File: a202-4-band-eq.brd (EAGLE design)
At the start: 100 x 50 mm, 71 parts, among them U1 SCREW-M2X8, U10 FX2-20S-1.27DS, U2 SCREW-M2X8, U3 NUT-M2-SELFLOCK, U4 NUT-M2-SELFLOCK, U5 FX2-20P-1.27DS, U6 SCREW-M2X8, U7 SCREW-M2X8, U8 NUT-M2-SELFLOCK, U9 NUT-M2-SELFLOCK

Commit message: Add Potentiometer Knobs
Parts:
- added O1, O2, O3, O4: 450-AA150(15MM,D,BLACK), hardware:EMPTY
- added O5, O6, O7, O8: 450-CP153(15MM,BLUE/WHITE), hardware:EMPTY
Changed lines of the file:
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@@
 <attribute name="MOUSER" value="81-RCER71H104K0A2H3B" x="12" y="-171" size="1.778" layer="27" display="off"/>
+</element>
+<element name="O1" library="hardware" package="EMPTY" value="450-AA150(15MM,D,BLACK)" x="-8" y="-109.25">
+<attribute name="MOUSER" value="450-AA150" x="-8" y="-109.25" size="1.778" layer="27" display="off"/>
+</element>
+<element name="O2" library="hardware" package="EMPTY" value="450-AA150(15MM,D,BLACK)" x="-9" y="-110.5">
+<attribute name="MOUSER" value="450-AA150" x="-9" y="-110.5" size="1.778" layer="27" display="off"/>
+</element>
+<element name="O3" library="hardware" package="EMPTY" value="450-AA150(15MM,D,BLACK)" x="-10" y="-111.75">
+<attribute name="MOUSER" value="450-AA150" x="-10" y="-111.75" size="1.778" layer="27" display="off"/>
+</element>
+<element name="O4" library="hardware" package="EMPTY" value="450-AA150(15MM,D,BLACK)" x="-11" y="-113">
+<attribute name="MOUSER" value="450-AA150" x="-11" y="-113" size="1.778" layer="27" display="off"/>
+</element>
+<element name="O5" library="hardware" package="EMPTY" value="450-CP153(15MM,BLUE/WHITE)" x="-12" y="-114.25">
+<attribute name="MOUSER" value="450-CP153" x="-12" y="-114.25" size="1.778" layer="27" display="off"/>
+</element>
+<element name="O6" library="hardware" package="EMPTY" value="450-CP153(15MM,BLUE/WHITE)" x="-13" y="-115.5">
+<attribute name="MOUSER" value="450-CP153" x="-13" y="-115.5" size="1.778" layer="27" display="off"/>
+</element>
+<element name="O7" library="hardware" package="EMPTY" value="450-CP153(15MM,BLUE/WHITE)" x="-14" y="-116.75">
+<attribute name="MOUSER" value="450-CP153" x="-14" y="-116.75" size="1.778" layer="27" display="off"/>
+</element>
+<element name="O8" library="hardware" package="EMPTY" value="450-CP153(15MM,BLUE/WHITE)" x="-15" y="-118">
+<attribute name="MOUSER" value="450-CP153" x="-15" y="-118" size="1.778" layer="27" display="off"/>
 </element>
 </elements>

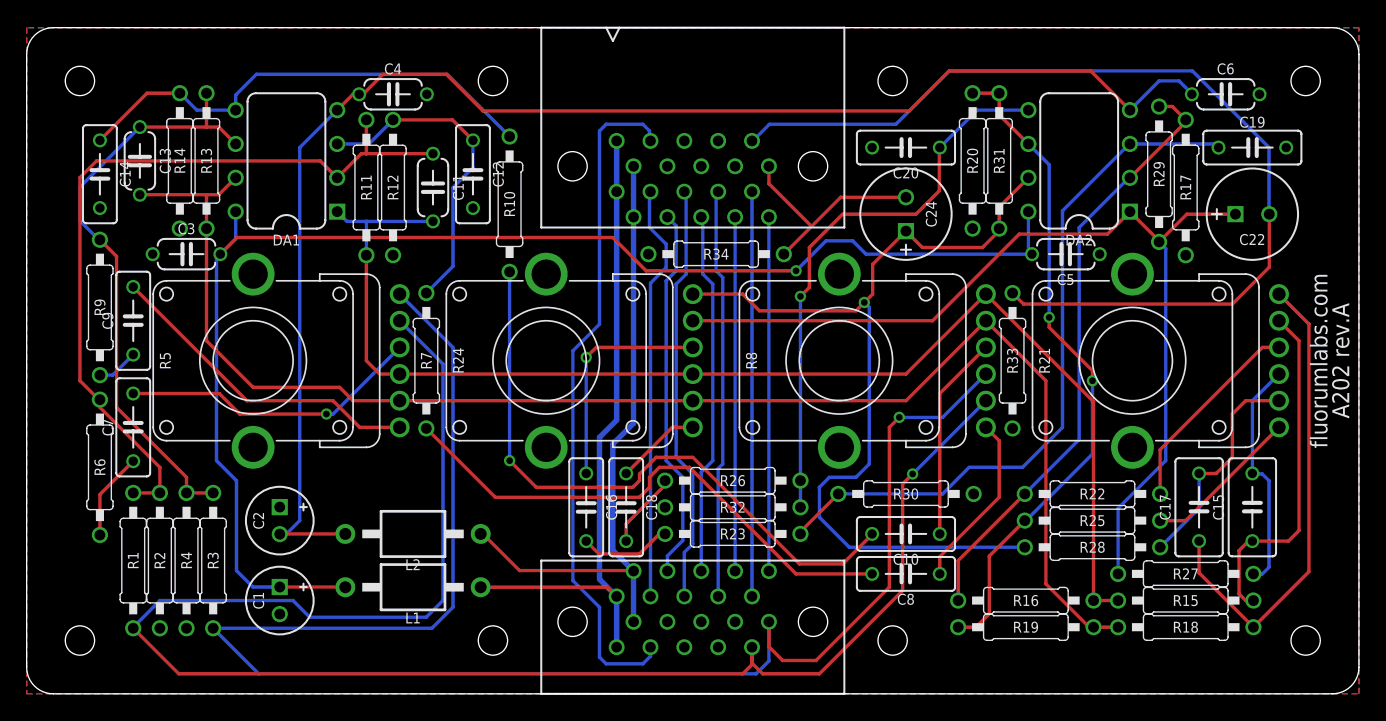
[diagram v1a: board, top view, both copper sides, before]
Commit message: PCB Update
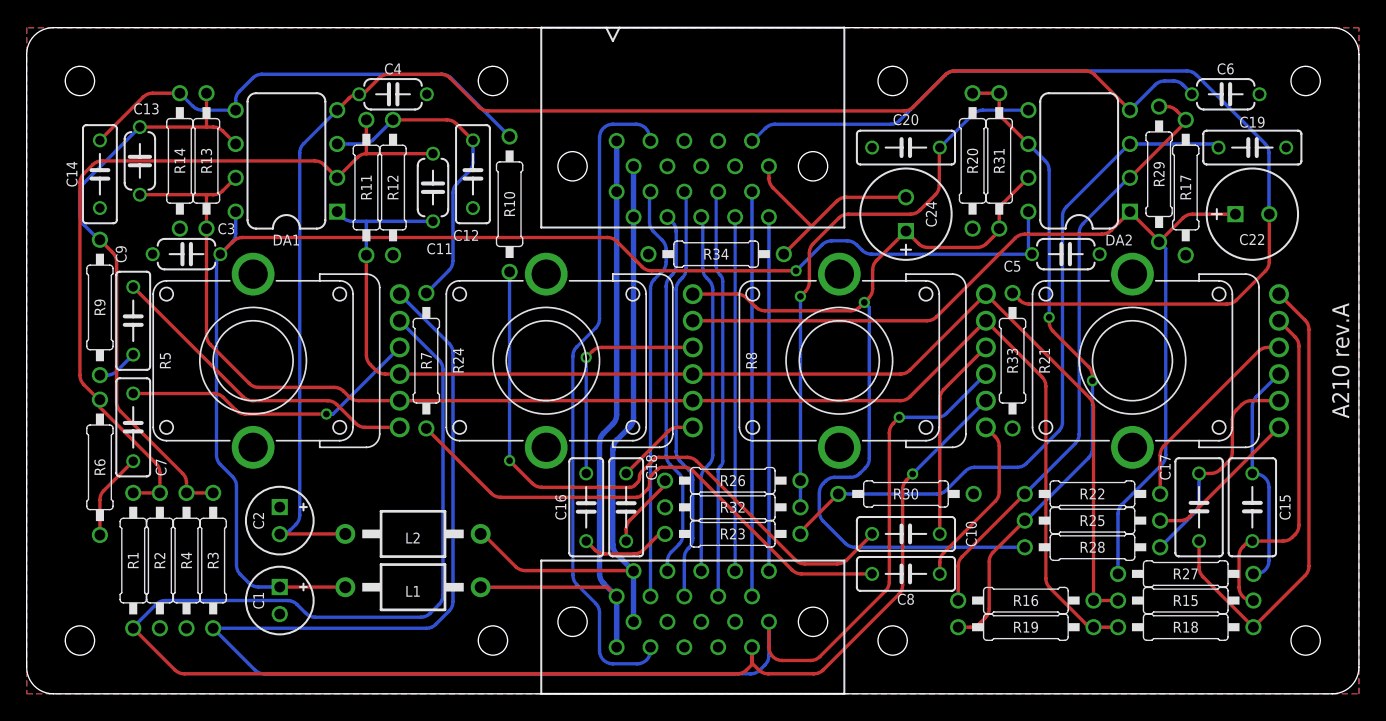
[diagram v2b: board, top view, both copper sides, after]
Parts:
- PCB1: value A202 rev.A -> A210 rev.A
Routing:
- net N$7: track 51.0 -> 49.7 mm
- net N$37: track 68.6 -> 67.7 mm
- net N$47: track 109.0 -> 108.2 mm
- net N$14: track 129.3 -> 128.5 mm
- net N$45: track 104.0 -> 103.2 mm
- net N$23: track 17.6 -> 17.0 mm
- net N$32: track 124.8 -> 124.2 mm
- net N$29: track 109.9 -> 109.4 mm
- net N$24: track 26.0 -> 25.5 mm
- net N$27: track 73.1 -> 72.6 mm
- net N$36: track 50.0 -> 49.5 mm
